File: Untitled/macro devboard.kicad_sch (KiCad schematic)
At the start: 50 parts, among them J1 12402012E212A, J3 Conn_02x13_Counter_Clockwise, SW1 MX_SW_HS, SW2 MX_SW_HS, SW3 RST, SW6 MX_SW_HS, SW7 MX_SW_HS, SW8 MX_SW_HS, SW9 MX_SW_HS, U2 ATmega32U4-A, Y2 ABM8-16.000MHz-D1X-T

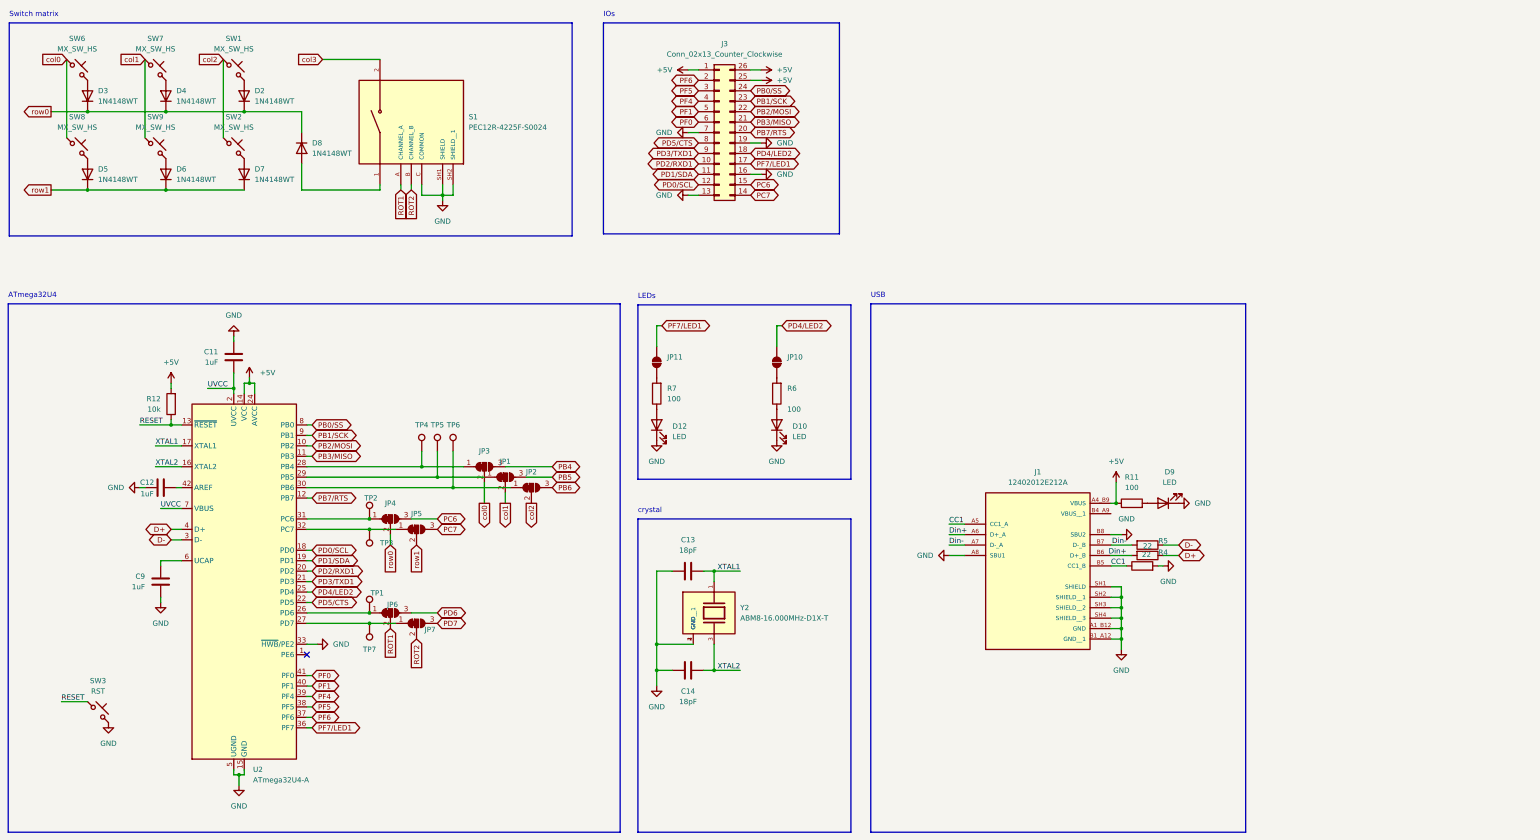
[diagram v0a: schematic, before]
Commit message: yes
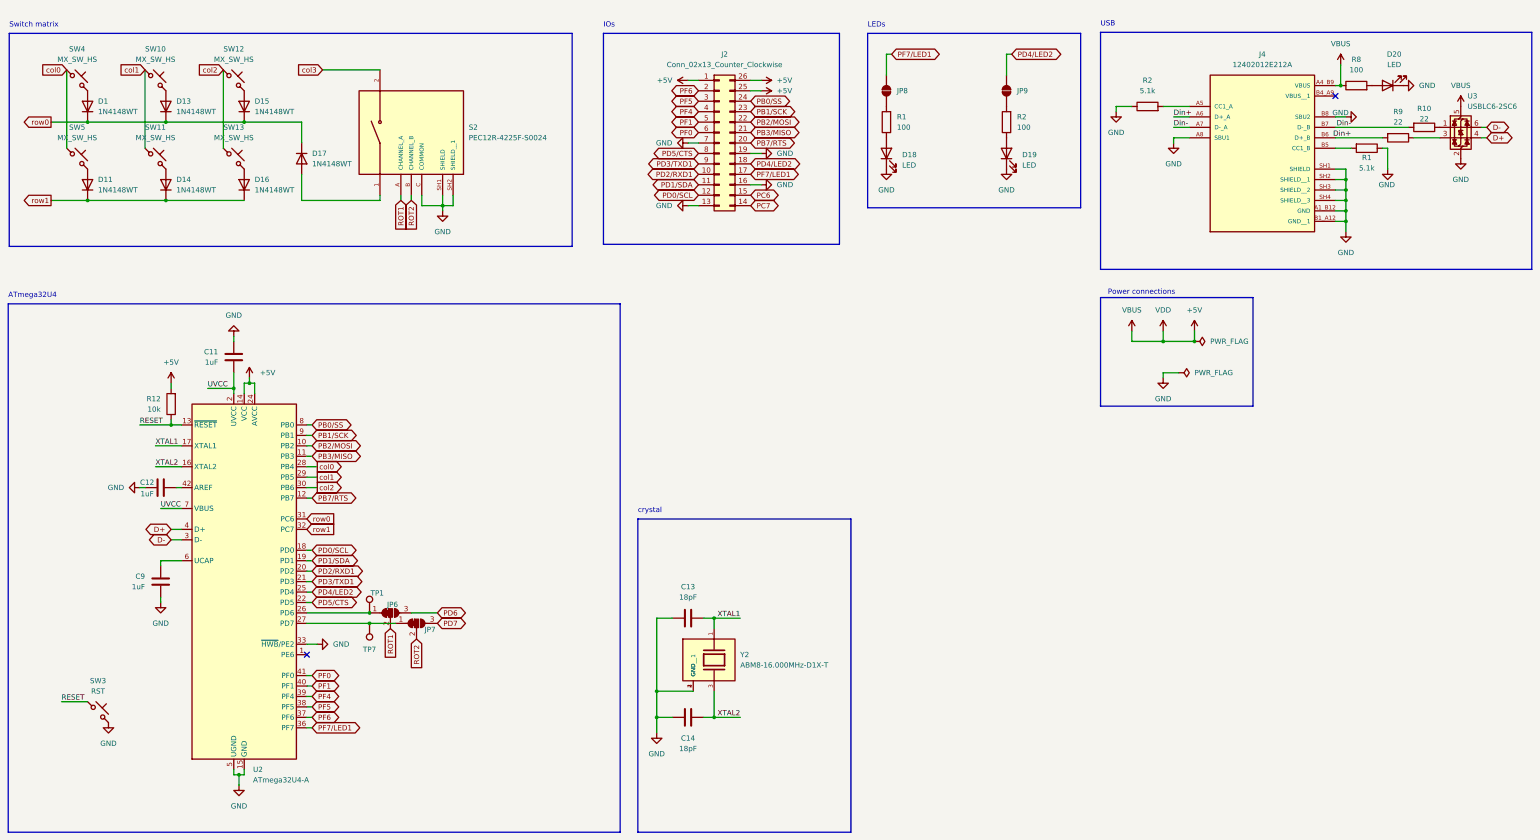
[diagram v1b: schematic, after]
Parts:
- removed D10, D12, D9: LED, LED_SMD:LED_0603_1608Metric_Pad1.05x0.95mm_HandSolder, symbol Device:LED
- removed D2, D3, D4, D5, D6, D7, D8: 1N4148WT, Diode_SMD:D_SOD-323F, symbol Diode:1N4148WT
- removed J1: 12402012E212A, 12402012E212A:AMPHENOL_12402012E212A, symbol 12402012E212A:12402012E212A
- removed J3: Conn_02x13_Counter_Clockwise, Connector_PinHeader_2.54mm:PinHeader_2x13_P2.54mm_Vertical, symbol Connector_Generic:Conn_02x13_Counter_Clockwise
- removed JP1, JP2, JP3, JP4, JP5: SolderJumper_3_Bridged12, Jumper:SolderJumper-3_P1.3mm_Bridged12_RoundedPad1.0x1.5mm_NumberLabels, symbol Jumper:SolderJumper_3_Bridged12
- removed JP10, JP11: SolderJumper_2_Open, Jumper:SolderJumper-2_P1.3mm_Open_RoundedPad1.0x1.5mm, symbol Jumper:SolderJumper_2_Open
- removed R11, R6, R7: 100, Resistor_SMD:R_0805_2012Metric_Pad1.20x1.40mm_HandSolder, symbol Device:R
- removed R3: 4.7k, Resistor_SMD:R_0805_2012Metric_Pad1.20x1.40mm_HandSolder, symbol Device:R
- removed R4, R5: 22, Resistor_SMD:R_0805_2012Metric_Pad1.20x1.40mm_HandSolder, symbol Device:R
- removed S1: PEC12R-4225F-S0024, PEC12R_4225F_S0024:XDCR_PEC12R-4225F-S0024, symbol PEC12R-4225F-S0024:PEC12R-4225F-S0024
- removed SW1, SW2, SW6, SW7, SW8, SW9: MX_SW_HS, keyswitches:Kailh_socket_MX, symbol PCM_marbastlib-mx:MX_SW_HS
- removed TP2, TP3, TP4, TP5, TP6: TestPoint, Connector_PinHeader_2.54mm:PinHeader_1x01_P2.54mm_Vertical, symbol Connector:TestPoint
- added D1, D11, D13, D14, D15, D16, D17: 1N4148WT, Diode_SMD:D_SOD-323F, symbol Diode:1N4148WT
- added D18, D19, D20: LED, LED_SMD:LED_0603_1608Metric_Pad1.05x0.95mm_HandSolder, symbol Device:LED
- added J2: Conn_02x13_Counter_Clockwise, Connector_PinHeader_2.54mm:PinHeader_2x13_P2.54mm_Vertical, symbol Connector_Generic:Conn_02x13_Counter_Clockwise
- added J4: 12402012E212A, 12402012E212A:AMPHENOL_12402012E212A, symbol 12402012E212A:12402012E212A
- added JP8, JP9: SolderJumper_2_Open, Jumper:SolderJumper-2_P1.3mm_Open_RoundedPad1.0x1.5mm, symbol Jumper:SolderJumper_2_Open
- added R1, R2: 5.1k, Resistor_SMD:R_0805_2012Metric_Pad1.20x1.40mm_HandSolder, symbol Device:R
- added R1, R2, R8: 100, Resistor_SMD:R_0805_2012Metric_Pad1.20x1.40mm_HandSolder, symbol Device:R
- added R10, R9: 22, Resistor_SMD:R_0805_2012Metric_Pad1.20x1.40mm_HandSolder, symbol Device:R
- added S2: PEC12R-4225F-S0024, PEC12R_4225F_S0024:XDCR_PEC12R-4225F-S0024, symbol PEC12R-4225F-S0024:PEC12R-4225F-S0024
- added SW10, SW11, SW12, SW13, SW4, SW5: MX_SW_HS, keyswitches:Kailh_socket_MX, symbol PCM_marbastlib-mx:MX_SW_HS
- added U3: USBLC6-2SC6, Package_TO_SOT_SMD:SOT-23-6_Handsoldering, symbol Power_Protection:USBLC6-2SC6
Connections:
- net +5V: now also J2.1 (Pin_1), J2.25 (Pin_25), J2.26 (Pin_26), J4.A4_B9 (VBUS), R8.1, U3.5 (VBUS)
- net D+: now also U3.4 (I/O2)
- net D-: now also U3.6 (I/O1)
- net Din+: now also J4.A6 (D+_A), J4.B6 (D+_B), R9.2
- net Din-: now also J4.A7 (D-_A), J4.B7 (D-_B), R10.2
- net GND: now also D18.1 (K), D19.1 (K), D20.1 (K), J2.13 (Pin_13), J2.16 (Pin_16), J2.19 (Pin_19), J2.7 (Pin_7), J4.A1_B12 (GND), J4.A8 (SBU1), J4.B1_A12 (GND__1), J4.B8 (SBU2), J4.SH1 (SHIELD), J4.SH2 (SHIELD__1), J4.SH3 (SHIELD__2), J4.SH4 (SHIELD__3), R1.1, R2.1, S2.C (COMMON), S2.SH1 (SHIELD), S2.SH2 (SHIELD__1), U3.2 (GND)
- net PB0/SS: now also J2.24 (Pin_24)
- net PB1/SCK: now also J2.23 (Pin_23)
- net PB2/MOSI: now also J2.22 (Pin_22)
- net PB3/MISO: now also J2.21 (Pin_21)
- net PB7/RTS: now also J2.20 (Pin_20)
- net PC6: now also J2.15 (Pin_15)
- net PC7: now also J2.14 (Pin_14)
- net PD0/SCL: now also J2.12 (Pin_12)
- net PD1/SDA: now also J2.11 (Pin_11)
- net PD2/RXD1: now also J2.10 (Pin_10)
- net PD3/TXD1: now also J2.9 (Pin_9)
- net PD4/LED2: now also J2.18 (Pin_18), JP9.2 (B)
- net PD5/CTS: now also J2.8 (Pin_8)
- net PF0: now also J2.6 (Pin_6)
- net PF1: now also J2.5 (Pin_5)
- net PF4: now also J2.4 (Pin_4)
- net PF5: now also J2.3 (Pin_3)
- net PF6: now also J2.2 (Pin_2)
- net PF7/LED1: now also J2.17 (Pin_17), JP8.2 (B)
- net ROT1: now also S2.A (CHANNEL_A)
- net ROT2: now also S2.B (CHANNEL_B)
- net col0: now also U2.28 (PB4), SW4.1, SW5.1
- net col1: now also U2.29 (PB5), SW10.1, SW11.1
- net col2: now also U2.30 (PB6), SW12.1, SW13.1
- net col3: now also S2.2
- net row0: now also U2.31 (PC6), D1.1 (K), D13.1 (K), D15.1 (K), D17.1 (K)
- net row1: now also U2.32 (PC7), D11.1 (K), D14.1 (K), D16.1 (K)
- new net: R9.1, U3.3 (I/O2)
- new net: D15.2 (A), SW12.2
- new net: D1.2 (A), SW4.2
- new net: J4.A5 (CC1_A), R2.2
- new net: J4.B5 (CC1_B), R1.2
- new net: JP8.1 (A), R1.2
- new net: D19.2 (A), R2.1
- new net: D16.2 (A), SW13.2
- new net: JP9.1 (A), R2.2
- new net: D20.2 (A), R8.2
- new net: D14.2 (A), SW11.2
- new net: D11.2 (A), SW5.2
- new net: D18.2 (A), R1.1
- new net: D13.2 (A), SW10.2
- new net: R10.1, U3.1 (I/O1)
- new net: D17.2 (A), S2.1
- no-connect marks 1 -> 2
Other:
- note added: "Power connections"
- moved on the sheet: C13, C14, Y2
